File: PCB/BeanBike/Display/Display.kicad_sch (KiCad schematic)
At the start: 4 parts, among them J1 Pi 0 2W, J2 Power Conn, J3 Data Conn, J5 Display Conn

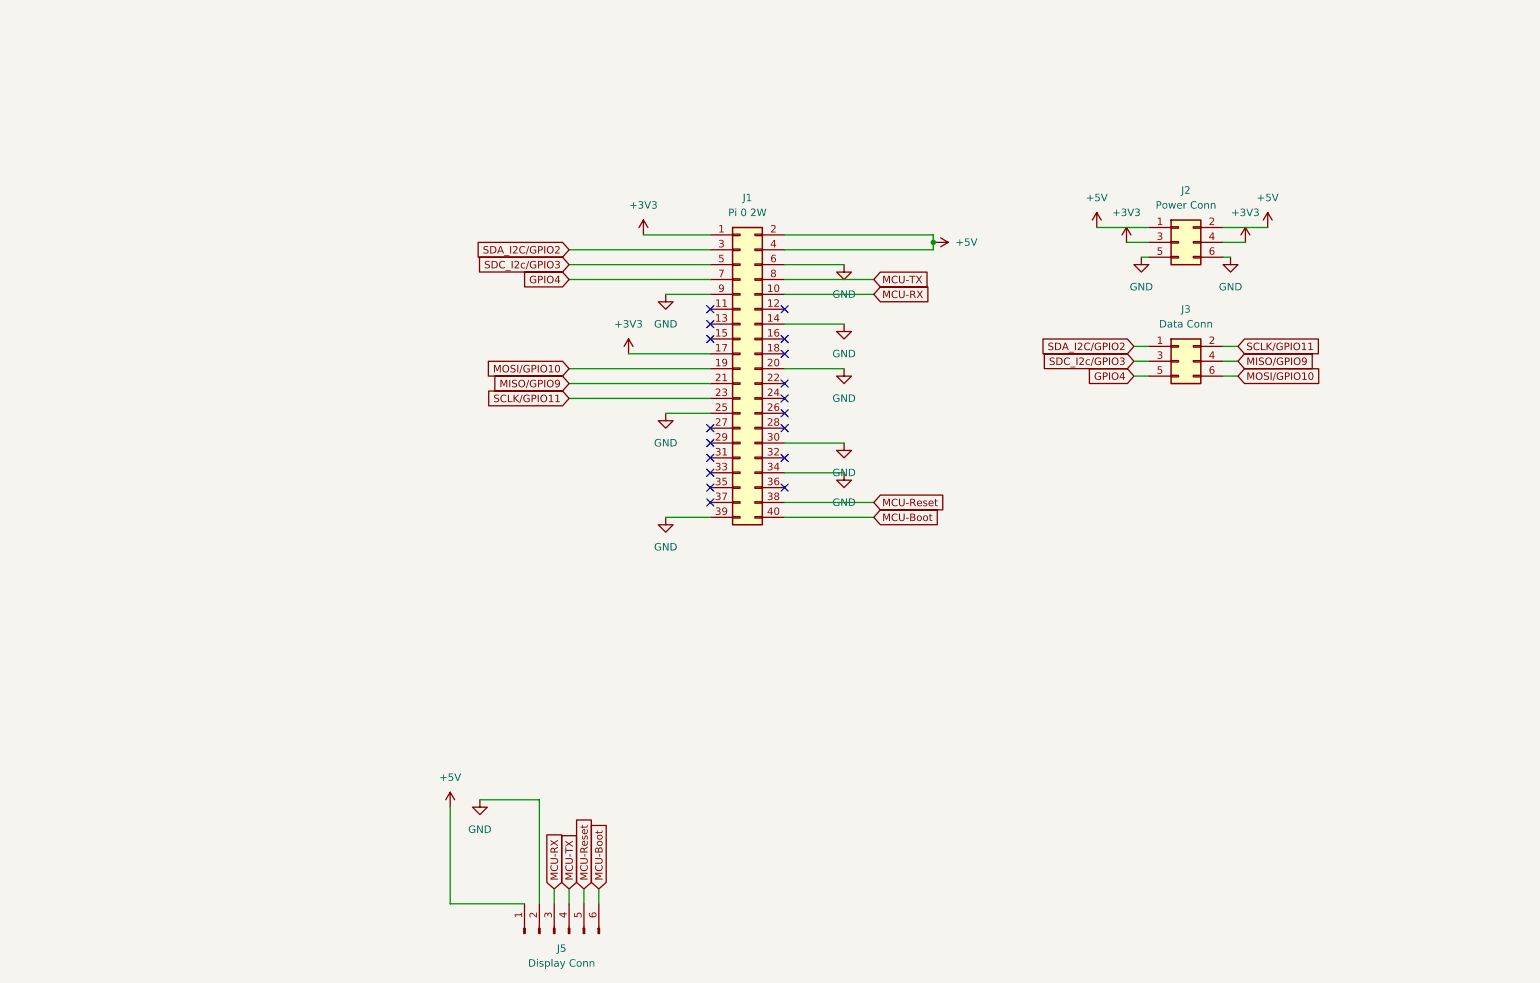
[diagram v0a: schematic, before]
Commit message: Finish up
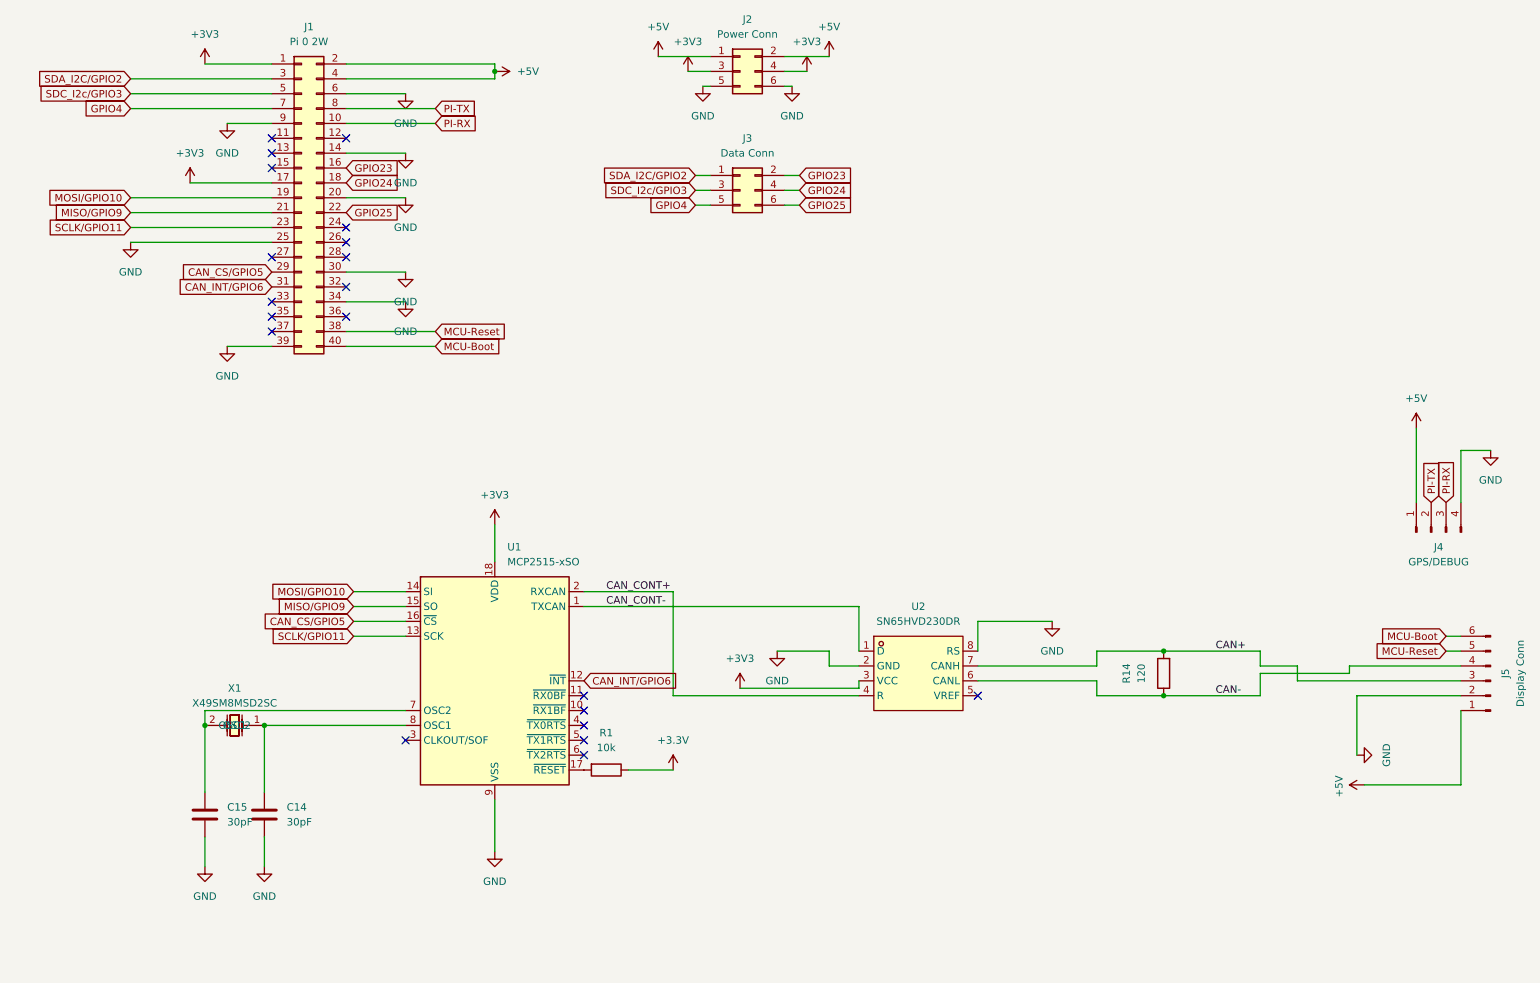
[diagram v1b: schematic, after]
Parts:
- added C14, C15: 30pF, Capacitor_SMD:C_0402_1005Metric, symbol Device:C
- added J4: GPS/DEBUG, Connector_PinHeader_2.54mm:PinHeader_1x04_P2.54mm_Vertical, symbol Connector:Conn_01x04_Pin
- added R1: 10k, Resistor_SMD:R_0805_2012Metric, symbol Device:R
- added R14: 120, Resistor_SMD:R_0805_2012Metric, symbol Device:R
- added U1: MCP2515-xSO, Package_SO:SOIC-18W_7.5x11.6mm_P1.27mm, symbol Interface_CAN_LIN:MCP2515-xSO
- added U2: SN65HVD230DR, easyeda2kicad:SOIC-8_L4.9-W3.9-P1.27-LS6.0-BL, symbol easyeda2kicad:SN65HVD230DR
- added X1: X49SM8MSD2SC, easyeda2kicad:CRYSTAL-SMD_L11.5-W4.8-LS12.7, symbol easyeda2kicad:X49SM8MSD2SC
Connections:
- net +3V3: now also U1.18 (VDD), U2.3 (VCC)
- net +5V: now also J4.1 (Pin_1)
- net GND: now also C14.2, C15.2, J4.4 (Pin_4), U1.9 (VSS), U2.2 (GND), U2.8 (RS)
- net MISO/GPIO9: now also U1.15 (SO); no longer J3.4 (Pin_4)
- net MOSI/GPIO10: now also U1.14 (SI); no longer J3.6 (Pin_6)
- net SCLK/GPIO11: now also U1.13 (SCK); no longer J3.2 (Pin_2)
- net GPIO23: now reaches J1.16 (Pin_16)
- net GPIO23: now also J3.2 (Pin_2)
- net GPIO24: now reaches J1.18 (Pin_18)
- net GPIO24: now also J3.4 (Pin_4)
- net GPIO25: now reaches J1.22 (Pin_22)
- net GPIO25: now also J3.6 (Pin_6)
- net CAN_CS/GPIO5: now reaches J1.29 (Pin_29)
- net CAN_CS/GPIO5: now also U1.16 (~{CS})
- net CAN_INT/GPIO6: now reaches J1.31 (Pin_31)
- net CAN_INT/GPIO6: now also U1.12 (~{INT})
- net MCU-RX renamed CAN+
- net CAN+: now also R14.2, U2.7 (CANH); no longer J1.10 (Pin_10)
- net MCU-TX renamed CAN-
- net CAN-: now also R14.1, U2.6 (CANL); no longer J1.8 (Pin_8)
- new net: R1.2, U1.17 (~{RESET})
- new net: C15.1, U1.7 (OSC2), X1.2 (OSC2)
- new net: C14.1, U1.8 (OSC1), X1.1 (OSC1)
- new net +3.3V: R1.1
- new net CAN_CONT+: U1.2 (RXCAN), U2.4 (R)
- new net CAN_CONT-: U1.1 (TXCAN), U2.1 (D)
- new net PI-RX: J1.10 (Pin_10), J4.3 (Pin_3)
- new net PI-TX: J1.8 (Pin_8), J4.2 (Pin_2)
- no-connect marks 18 -> 20
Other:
- moved on the sheet: J1, J2, J3, J5
